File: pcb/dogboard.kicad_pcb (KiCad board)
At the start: 2 copper layers, 45.1 x 32.6 mm, 30 parts, among them J1 Barrel_Jack_Switch_Pin3Ring, J2 qtpy1, J3 Conn_01x02_Male, Q1 MMBT3904, Q2 MMBT3904, SW1 SW_Push, U1 LD1117S50TR_SOT223, U2 LM555xN

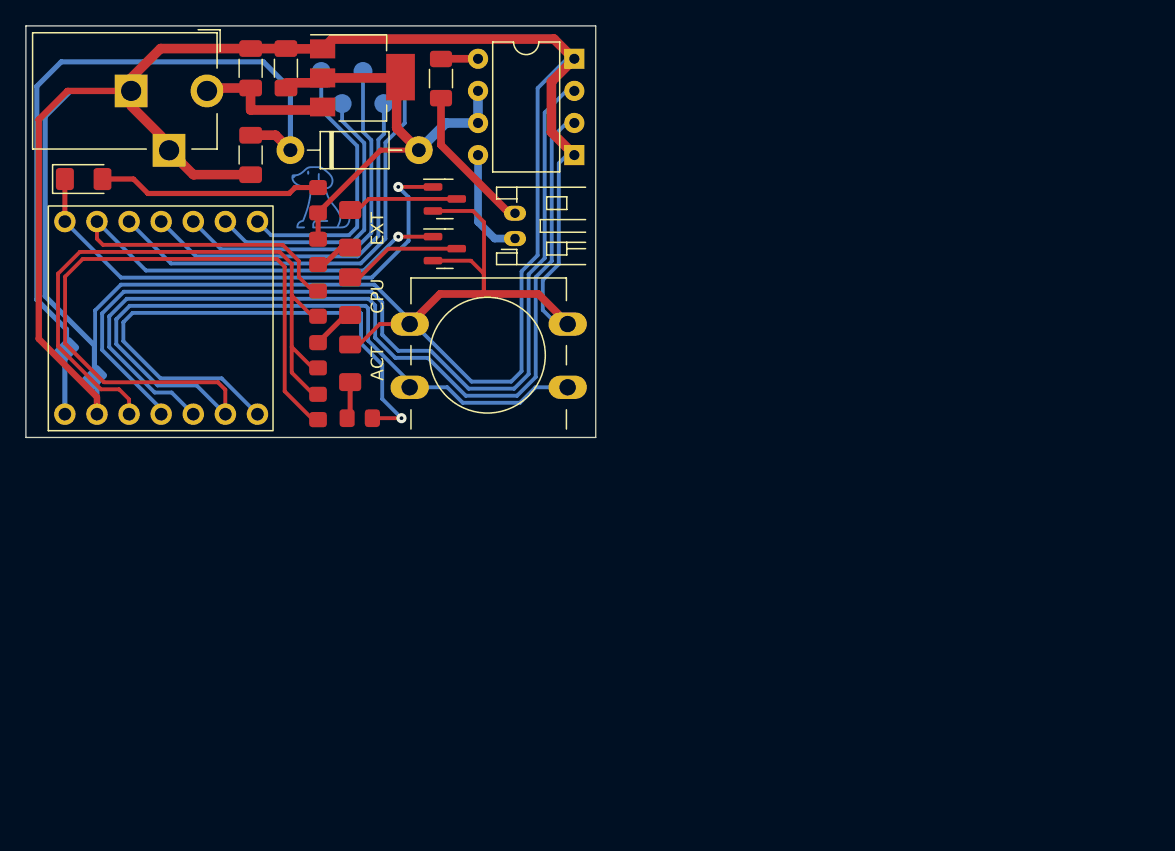
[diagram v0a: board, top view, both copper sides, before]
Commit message: pcb refactor
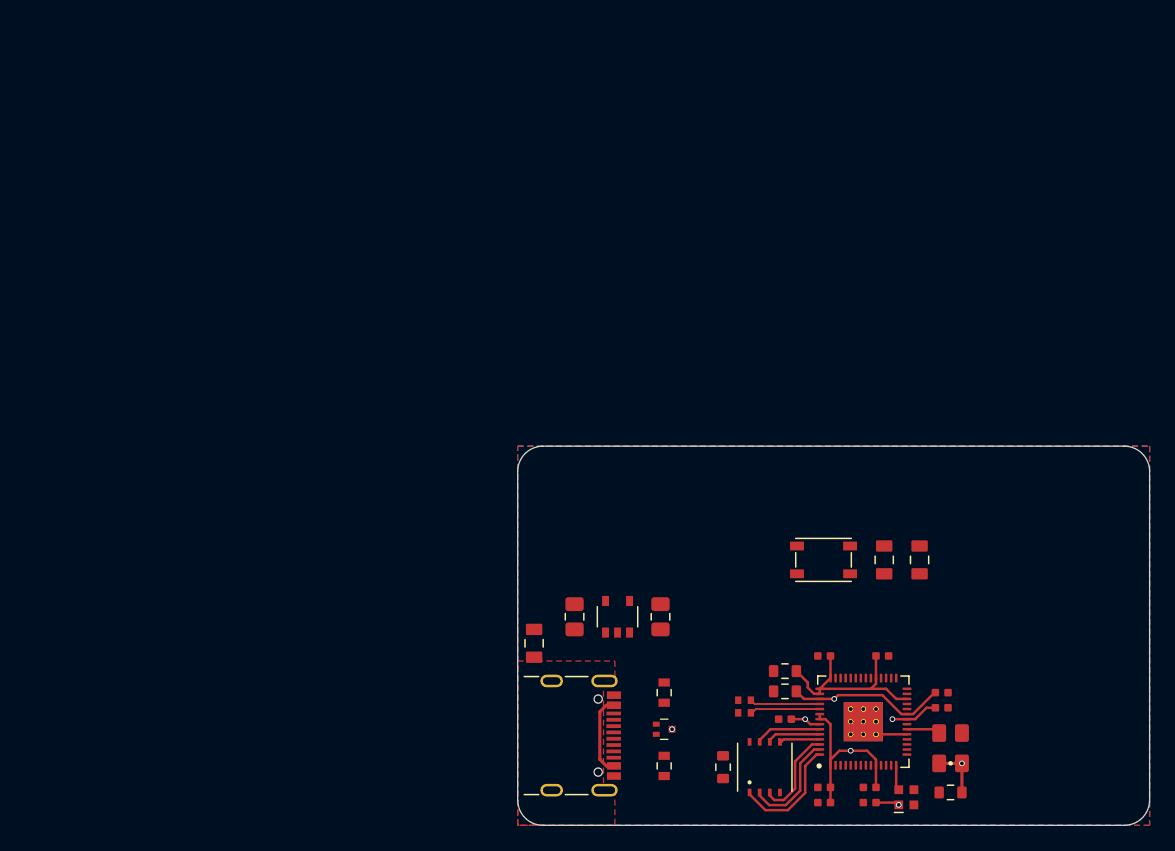
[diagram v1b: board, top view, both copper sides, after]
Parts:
- removed C3: 1uF, Capacitor_SMD:C_1206_3216Metric_Pad1.33x1.80mm_HandSolder
- removed D2: D_Schottky, Diode_SMD:D_1206_3216Metric_Pad1.42x1.75mm_HandSolder
- removed D3, D4, D5: LED, LED_SMD:LED_1206_3216Metric_Pad1.42x1.75mm_HandSolder
- removed J2: qtpy1, Module:qtpy1_reverse
- removed J3: Conn_01x02_Male, Connector_JST:JST_PH_S2B-PH-K_1x02_P2.00mm_Horizontal
- removed Q1, Q2: MMBT3904, Package_TO_SOT_SMD:SOT-23
- removed R5: 82, Resistor_SMD:R_0805_2012Metric_Pad1.20x1.40mm_HandSolder
- removed REF**: dog_better, proj_footprints:dog_better
- removed SW1: SW_Push, Button_Switch_THT:SW_PUSH-12mm
- removed TP3, TP4, TP5, TP6, TP7: TestPoint, TestPoint:TestPoint_Pad_D1.5mm
- removed U2: LM555xN, Package_DIP:DIP-8_W7.62mm
- added C10: 0.1u, _custom:CAP_0402_HandSolder, F.Cu at (151.8, 111.0)
- added C11: 0.1u, _custom:CAP_0402_HandSolder, F.Cu at (148.2, 100.6)
- added C12: 0.1u, _custom:CAP_0402_HandSolder, F.Cu at (148.2, 112.2)
- added C13: 0.1u, _custom:CAP_0402_HandSolder, F.Cu at (157.6, 104.7)
- added C14: 0.1u, _custom:CAP_0402_HandSolder, F.Cu at (152.8, 100.6)
- added C15: 0.1u, _custom:CAP_0402_HandSolder, F.Cu at (148.2, 111.0)
- added C18: 0.1u, _custom:CAP_0402_HandSolder, F.Cu at (151.8, 112.2)
- added C5: 0.1uF, _custom:CAP_0603_HandSolder, F.Cu at (158.2, 111.4)
- added C6: 1u, _custom:CAP_0603_HandSolder, F.Cu at (145.2, 103.4)
- added C7: 0.1u, _custom:CAP_0402_HandSolder, F.Cu at (145.2, 105.6)
- added C8: 0.1u, _custom:CAP_0402_HandSolder, F.Cu at (157.6, 103.5)
- added C9: 1u, _custom:CAP_0603_HandSolder, F.Cu at (145.2, 101.8)
- added D6: NeoPxl, _custom:LED_NeoPixel_0606, F.Cu at (154.8, 111.8)
- added R8: 27, _custom:R_0402_HandSolder, F.Cu at (141.9, 105.1)
- added REG1: 3.3v Linear, _custom:reg_SMD_SOT-25, F.Cu at (131.9, 97.5)
- added SW2: BOOT, _custom:button_SMD_PTS810, F.Cu at (148.2, 93.0)
- added U3: 4MB Flash, _custom:flash_SMD_XSON-8_4x4mm, F.Cu at (143.6, 109.4)
- added Y1: 12 MHz, _custom:XO_Osc_4-SMD_3.2x2.5, F.Cu at (158.2, 107.9)
- C1: footprint Capacitor_SMD:C_1206_3216Metric_Pad1.33x1.80mm_HandSolder -> _custom:CAP_0805_HandSolder
- C2: value 4.7 -> 1uF; footprint Capacitor_SMD:C_1206_3216Metric_Pad1.33x1.80mm_HandSolder -> _custom:CAP_0805_HandSolder
- C4: value 1uF -> 0.1u; footprint Capacitor_SMD:C_1206_3216Metric_Pad1.33x1.80mm_HandSolder -> _custom:CAP_0603_HandSolder
- D1: value SB130 -> ESD Protection; footprint Diode_THT:D_DO-41_SOD81_P10.16mm_Horizontal -> _custom:tvs_USB2_SOT-723
- J1: value Barrel_Jack_Switch_Pin3Ring -> USB-C / USB2.0; footprint Connector_BarrelJack:BarrelJack_CUI_PJ-102AH_Horizontal -> _custom:USB_C_Receptacle_SMD_GCT
- R1: value 47 -> 20k; footprint Resistor_SMD:R_0805_2012Metric_Pad1.20x1.40mm_HandSolder -> _custom:R_0805_HandSolder
- R2: value 10k -> 5.1k; footprint Resistor_SMD:R_0805_2012Metric_Pad1.20x1.40mm_HandSolder -> _custom:R_0603_HandSolder
- R3: value 220 -> 5.1k; footprint Resistor_SMD:R_0805_2012Metric_Pad1.20x1.40mm_HandSolder -> _custom:R_0603_HandSolder
- R4: footprint Resistor_SMD:R_0805_2012Metric_Pad1.20x1.40mm_HandSolder -> _custom:R_0805_HandSolder
- R6: value 150 -> 1k; footprint Resistor_SMD:R_1206_3216Metric_Pad1.30x1.75mm_HandSolder -> _custom:R_0805_HandSolder
- R7: value 10k -> 27; footprint Resistor_SMD:R_0805_2012Metric_Pad1.20x1.40mm_HandSolder -> _custom:R_0402_HandSolder
- U1: value LD1117S50TR_SOT223 -> RP2040; footprint Package_TO_SOT_SMD:SOT-223-3_TabPin2 -> _custom:RP2040_QFN-56
- moved U1 64.5 mm to (151.3, 105.8), turned to 90 degrees
- moved C4 61.2 mm to (140.2, 109.4)
- moved J1 58.4 mm to (127.8, 106.9)
- moved D1 54.5 mm to (135.6, 106.4)
- moved C1 54.2 mm to (135.3, 97.5)
- moved R2 52.5 mm to (135.6, 109.3)
- moved R6 51.8 mm to (153.0, 93.0), turned to -90 degrees
- moved R4 51.7 mm to (155.8, 93.0)
- moved C2 49.0 mm to (128.5, 97.5), turned to 90 degrees
- moved R3 44.3 mm to (135.6, 103.5)
- moved R7 41.0 mm to (141.9, 104.1), turned to 0 degrees
- moved R1 22.5 mm to (125.3, 99.6), turned to 90 degrees
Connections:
- C1 pad 2: Net-(C1-Pad2) -> VBUS
- C2 pad 2: Net-(C2-Pad2) -> +3.3V
- C4 pad 2: Net-(C3-Pad2) -> +3.3V
- D1 pad 1: Net-(C3-Pad2) -> /USB_D-
- D1 pad 2: Net-(C2-Pad2) -> /USB_D+
- R1 pad 1: Net-(J2-Pad14) -> GNDPWR
- R1 pad 2: Net-(D4-Pad2) -> GNDREF
- R2 pad 1: Net-(C2-Pad2) -> /CC2
- R2 pad 2: Net-(D2-Pad2) -> GNDREF
- R3 pad 1: Net-(C2-Pad2) -> /CC1
- R3 pad 2: Net-(D3-Pad2) -> GNDREF
- R4 pad 1: Net-(J2-Pad10) -> /~{BOOT}
- R4 pad 2: Net-(J2-Pad2) -> +3.3V
- R6 pad 2: Net-(R6-Pad2) -> /~{BOOT}
- R7 pad 1: Net-(J2-Pad13) -> /USB_D-
- R7 pad 2: Net-(J2-Pad10) -> /TR-
- U1 pad 1: GNDREF -> +3.3V
- U1 pad 2: Net-(C2-Pad2) -> GPIO0
- U1 pad 3: Net-(C1-Pad2) -> GPIO1
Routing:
- net GNDREF: track 248.0 -> 3.86 mm, vias 0 -> 1
- net Net-(J2-Pad13): track 107.5 -> 0.00 mm
- net Net-(J2-Pad11): track 73.8 -> 0.00 mm
- net Net-(J2-Pad12): track 72.6 -> 0.00 mm
- net Net-(C3-Pad2): track 57.2 -> 0.00 mm
- net Net-(J2-Pad10): track 50.8 -> 0.00 mm
- net Net-(J2-Pad2): track 50.6 -> 0.00 mm, vias 1 -> 0
- net Net-(J2-Pad14): track 45.6 -> 0.00 mm, vias 1 -> 0
- net Net-(D2-Pad1): track 40.9 -> 0.00 mm, vias 1 -> 0
- net +3.3V: track 0.00 -> 40.4 mm, vias 0 -> 4
- net Net-(J2-Pad3): track 36.3 -> 0.00 mm
- net Net-(C2-Pad2): track 36.2 -> 0.00 mm
- net Net-(J2-Pad4): track 29.6 -> 0.00 mm
- net Net-(J2-Pad5): track 28.6 -> 0.00 mm
- net Net-(J2-Pad6): track 22.8 -> 0.00 mm
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- added copper zone on F.Cu, net GNDPWR
- added copper zone on B.Cu, net GNDREF
- added copper zone on F.Cu, net GNDREF
- added copper zone on In1.Cu, net GNDREF
- added copper zone on In2.Cu, net GNDREF
- added copper zone on In3.Cu, net GNDREF
- added copper zone on In4.Cu, net GNDREF
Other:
- board size 45.1 x 32.6 mm -> 50 x 30 mm
- copper layers 2 -> 6
- board text removed: "ACT"
- board text removed: "CPU"
- board text removed: "DogBoard 1.0 BETA 2"
- board text removed: "EXT"
